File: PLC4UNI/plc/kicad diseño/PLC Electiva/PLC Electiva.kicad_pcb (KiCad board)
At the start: 2 copper layers, 102.4 x 83.1 mm, 177 parts, among them J1 Conn_02x08_Odd_Even, K1 G5V-1, K2 G5V-1, Q1 NCE60P04R, Q2 ZXMS6004FFQTA, Q3 ZXMS6004FFQTA, Q4 ZXMS6004FFQTA, Q5 ZXMS6004FFQTA, SW1 TS-1088-AR02016, U1 ESP32-S3-WROOM-1, U10 ADS1115IDGS, U11 AT3H4B-CUH-S, U12 AT3H4B-CUH-S, U13 LK1802, U14 AT3H4B-CUH-S, U15 MAX31856MUD+, U16 BL0942, U17 B0303S-1WR3_C7465185, U18 ISO7021DR, U2 AT3H4B-CUH-S, U3 AP63203WU, U4 RS485-PROTECT, U5 AT3H4B-CUH-S, U6 AT3H4B-CUH-S, U7 GP8211S-TC50-EW, U8 GP8302-TC50-EW, U9 BTS723GWXUMA1

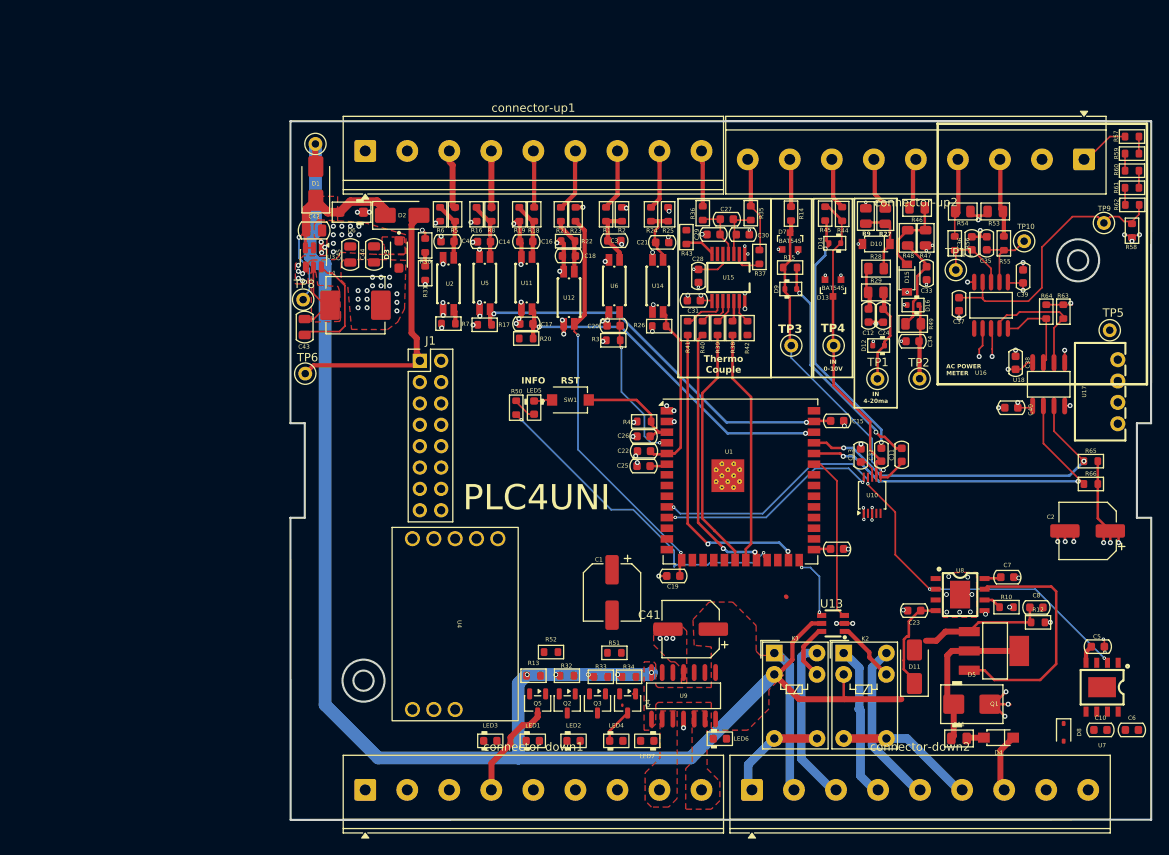
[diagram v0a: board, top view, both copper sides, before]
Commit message: Tamaños correctos
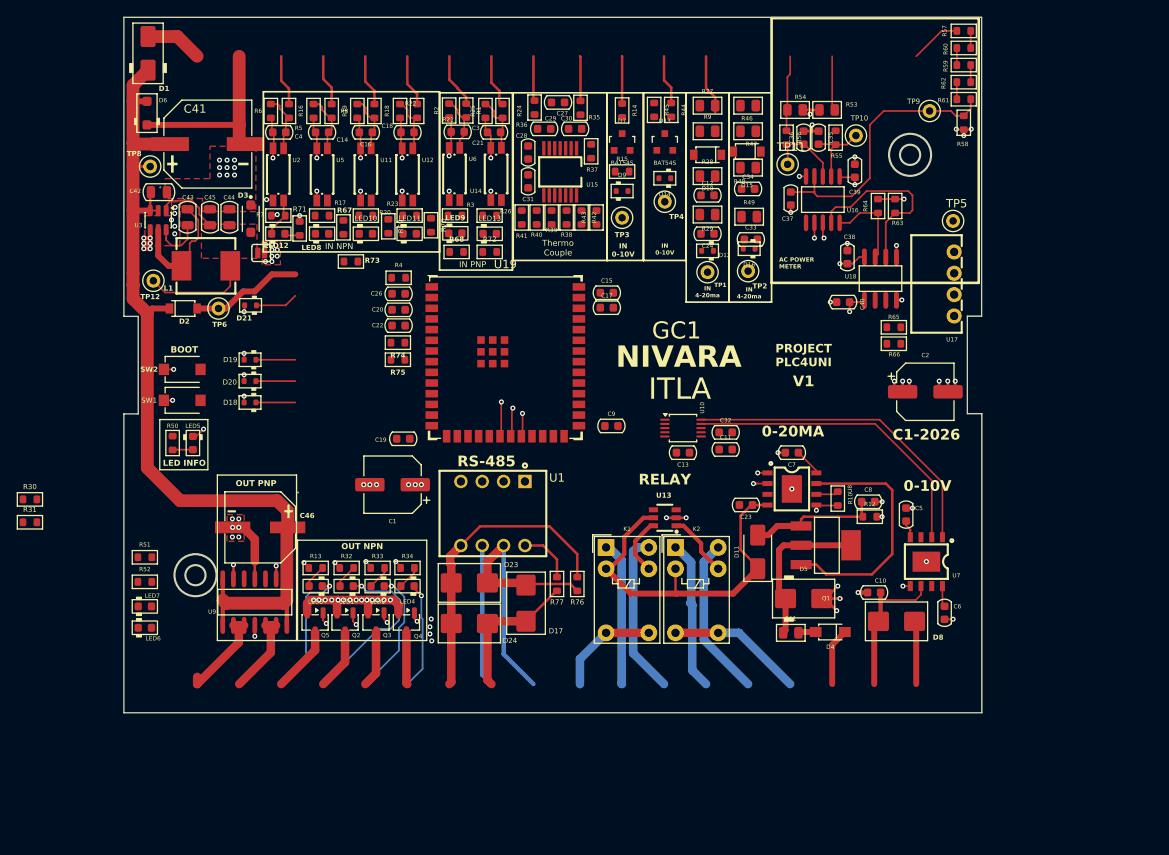
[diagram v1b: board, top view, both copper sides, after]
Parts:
- removed C25: 100nf, Capacitor_SMD_AKL:C_0603_1608Metric
- removed J1: Conn_02x08_Odd_Even, Connector_PinHeader_2.54mm:PinHeader_2x08_P2.54mm_Vertical
- removed TP7: TestPoint_Hole1, 4ms_TestPoint:TestPoint_WireHole
- removed U4: RS485-PROTECT, MG_footprints:RS-485-PROTECT
- removed connector-down1, connector-down2, connector-up1, connector-up2: Screw_Terminal_9_P5.00mm, TerminalBlock_Phoenix:TerminalBlock_Phoenix_PT-1,5-9-5.0-H_1x09_P5.00mm_Horizontal
- added C46: 100uF, EasyEDA:CAP-SMD_BD8.0-L8.3-W8.3-FD, F.Cu at (76.5, 95.8)
- added D17: SMBJ12CA, Diode_SMD_AKL:D_SMB_TVS, F.Cu at (108.1, 104.8)
- added D18: ESD5Z3.3T, Diode_SMD_AKL:D_SOD-523, F.Cu at (75.3, 80.9)
- added D19: ESD5Z3.3T, Diode_SMD_AKL:D_SOD-523, F.Cu at (75.3, 75.8)
- added D20: ESD5Z3.3T, Diode_SMD_AKL:D_SOD-523, F.Cu at (75.3, 78.4)
- added D21: ESD5Z3.3T, Diode_SMD_AKL:D_SOD-523, F.Cu at (75.4, 69.4)
- added D23: SMBJ6.5CA, Diode_SMD_AKL:D_SMB_TVS, F.Cu at (101.4, 102.4)
- added D24: SMBJ6.5CA, Diode_SMD_AKL:D_SMB_TVS, F.Cu at (101.4, 107.2)
- added JP1: ~, SparkFun-Jumper:Jumper_2_NO, F.Cu at (76.6, 63.1)
- added LED10: LED_0603_Red, LED_SMD_AKL:LED_0603_1608Metric, F.Cu at (89.1, 60.9)
- added LED11: LED_0603_Red, LED_SMD_AKL:LED_0603_1608Metric, F.Cu at (94.3, 60.9)
- added LED12: LED_0603_Red, LED_SMD_AKL:LED_0603_1608Metric, F.Cu at (78.7, 60.9)
- added LED13: LED_0603_Red, LED_SMD_AKL:LED_0603_1608Metric, F.Cu at (103.8, 60.9)
- added LED8: LED_0603_Red, LED_SMD_AKL:LED_0603_1608Metric, F.Cu at (83.9, 60.9)
- added LED9: LED_0603_Red, LED_SMD_AKL:LED_0603_1608Metric, F.Cu at (99.7, 60.8)
- added R67: R_0603, Resistor_SMD_AKL:R_0603_1608Metric, F.Cu at (86.4, 60.1)
- added R68: R_0603, Resistor_SMD_AKL:R_0603_1608Metric, F.Cu at (99.9, 63.0)
- added R69: R_0603, Resistor_SMD_AKL:R_0603_1608Metric, F.Cu at (91.7, 60.0)
- added R70: R_0603, Resistor_SMD_AKL:R_0603_1608Metric, F.Cu at (96.8, 59.8)
- added R71: R_0603, Resistor_SMD_AKL:R_0603_1608Metric, F.Cu at (81.2, 60.2)
- added R72: R_0603, Resistor_SMD_AKL:R_0603_1608Metric, F.Cu at (103.8, 63.0)
- added R73: 0R, Resistor_SMD_AKL:R_0603_1608Metric, F.Cu at (87.3, 64.2)
- added R74: 0R, Resistor_SMD_AKL:R_0603_1608Metric, F.Cu at (92.9, 73.8)
- added R75: 0R, Resistor_SMD_AKL:R_0603_1608Metric, F.Cu at (92.9, 75.8)
- added R76: 1K, Resistor_SMD_AKL:R_0603_1608Metric, F.Cu at (114.2, 102.5)
- added R77: 1K, Resistor_SMD_AKL:R_0603_1608Metric, F.Cu at (111.8, 102.5)
- added SW2: TS-1088-AR02016, EasyEDA:SW-SMD_L3.9-W3.0-P4.45, F.Cu at (67.2, 80.7)
- added TP12: TestPoint_Hole1, 4ms_TestPoint:TestPoint_WireHole, F.Cu at (63.8, 66.4)
- added U19: ESP32-S3-WROOM-1, Espressif:ESP32-S3-WROOM-1U, F.Cu at (105.7, 75.4)
- C41: value 47UF -> 220uF; footprint Capacitor_SMD:CP_Elec_6.3x7.7 -> EasyEDA:CAP-SMD_BD10.0-L10.3-W10.3-LS11.3-FD
- D1: value SS14 -> MBRA340T; footprint Diode_SMD:D_SMA -> Diode_SMD_AKL:D_SMA
- D2: value SS14 -> 1N5819HW-7-F; footprint Diode_SMD:D_SMA -> EasyEDA:SOD-123_L2.7-W1.6-LS3.7-RD
- D8: value SD12_SOD323 -> SMBJ12CA; footprint Diode_SMD:D_SOD-323 -> Diode_SMD_AKL:D_SMB_TVS
- L1: value 10uH -> APH0630T4R7M; footprint Inductor_SMD:L_APV_APH0630 -> EasyEDA:IND-SMD_L7.0-W6.6_APH0630
- R30, R31: value R_0603 -> 10K
- R4: value 22K -> 1K
- U1: value ESP32-S3-WROOM-1 -> TD301M485_C5451847; footprint RF_Module:ESP32-S3-WROOM-1U -> EasyEDA:COMM-TH_TD301M485
- moved C41 81.4 mm to (70.3, 50.2), turned to 0 degrees
- moved LED6 69.7 mm to (62.8, 107.7)
- moved LED7 61.9 mm to (62.8, 105.2), turned to 0 degrees
- moved R51 57.0 mm to (62.8, 99.3)
- moved R30 55.9 mm to (49.1, 92.4), turned to 0 degrees
- moved R31 55.6 mm to (49.1, 95.2), turned to 0 degrees
- moved U9 52.2 mm to (75.9, 104.7)
- moved R52 49.0 mm to (62.8, 102.3)
- moved SW1 46.3 mm to (67.2, 77.0), turned to 0 degrees
- moved R50 41.1 mm to (66.1, 85.7), turned to 90 degrees
- moved LED5 40.8 mm to (68.5, 85.7)
- moved C19 36.0 mm to (93.5, 85.2)
- moved R4 33.8 mm to (93.0, 66.1), turned to 0 degrees
- moved C26 33.7 mm to (93.0, 68.0)
- moved C22 32.8 mm to (93.0, 71.8)
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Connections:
- C14 pad 2: +24V -> VDC
- C16 pad 2: +24V -> VDC
- C18 pad 2: +24V -> VDC
- C23 pad 1: +24V -> VDC
- C4 pad 2: +24V -> VDC
- C41 pad 1: +24V -> VDC
- C42 pad 1: /PowerSupply/vdc_in -> VDC
- C44 pad 1: +3.3V -> /PowerSupply/ps_out
- C45 pad 1: +3.3V -> /PowerSupply/ps_out
- C5 pad 1: +24V -> VDC
- D1 pad 1: /PowerSupply/vdc_in -> VDC
- D11 pad 1: +24V -> VDC
- D2 pad 1: /PowerSupply/vdc_in -> VDC
- D3 pad A: +3.3V -> /PowerSupply/ps_out
- D6 pad 2: /PowerSupply/vdc_in -> VDC
- K1 pad 2: +24V -> VDC
- K2 pad 2: +24V -> VDC
- L1 pad 2: +3.3V -> /PowerSupply/ps_out
- R13 pad 1: +24V -> +3.3V
- R16 pad 1: +24V -> VDC
- R19 pad 1: +24V -> VDC
- R22 pad 1: +24V -> VDC
- R30 pad 1: +24V -> +3.3V
- R30 pad 2: /control/IN_VDC_ADC -> /control/RS485-RX
- R31 pad 1: /control/IN_VDC_ADC -> +3.3V
- R31 pad 2: GND -> /control/RS485-TX
- R32 pad 1: +24V -> +3.3V
- R33 pad 1: +24V -> +3.3V
- R34 pad 1: +24V -> +3.3V
- R38 pad 2: /control/mosi -> /control/SPI_MOSI
- R39 pad 2: /control/miso -> /control/SPI_MISO
- R4 pad 1: /control/EN -> +3.3V
- R4 pad 2: +3.3V -> /control/EN
- R40 pad 2: /control/clk -> /control/SPI_CLK
- R42 pad 2: /control/TC//FAULT -> /control/TC_FAULT
- R6 pad 1: +24V -> VDC
- SW1 pad 1: /control/EN -> GND
- SW1 pad 2: GND -> /control/IN_NPN1
- TP8 pad 1: /PowerSupply/vdc_in -> VDC
- U1 pad 1: GND -> /control/RS485-RX
- U1 pad 2: +3.3V -> /control/RS485-TX
- U1 pad 3: /control/EN -> GND
- U1 pad 4: /control/IN_PNP1 -> +3.3V
- U1 pad 5: /control/IN_PNP2 -> /control/CON_RS485_G
- U1 pad 6: /control/IN_VDC_ADC -> /control/CON_RS485_B
- U1 pad 7: /control/acc_cs -> /control/CON_RS485_A
- U1 pad 8: /control/GPIO1 -> Net-(U1-VO)
- U10 pad 10: /control/i2c_scl -> /control/I2C_SCK
- U10 pad 9: /control/i2c_sda -> /control/I2C_SDA
- U11 pad 2: +24V -> VDC
- U12 pad 2: +24V -> VDC
- U13 pad 5: +24V -> VDC
- U2 pad 2: +24V -> VDC
- U3 pad 1: +3.3V -> /PowerSupply/ps_out
- U3 pad 2: /PowerSupply/vdc_in -> VDC
- U3 pad 3: /PowerSupply/vdc_in -> VDC
- U5 pad 2: +24V -> VDC
- U7 pad 1: /control/i2c_scl -> /control/I2C_SCK
- U7 pad 2: /control/i2c_sda -> /control/I2C_SDA
- U7 pad 4: +24V -> VDC
- U8 pad 1: /control/i2c_scl -> /control/I2C_SCK
- U8 pad 2: /control/i2c_sda -> /control/I2C_SDA
- U8 pad 4: +24V -> VDC
- U9 pad 1: +24V -> VDC
- U9 pad 14: +24V -> VDC
- U9 pad 7: +24V -> VDC
- U9 pad 8: +24V -> VDC
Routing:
- net +24V: track 216.0 -> 6.82 mm, vias 16 -> 0
- net VDC: track 0.00 -> 179.3 mm, vias 0 -> 4
- net /control/i2c_sda: track 69.9 -> 0.00 mm, vias 4 -> 0
- net /control/IN_NPN4: track 48.7 -> 0.00 mm, vias 2 -> 0
- net /control/IN_NPN2: track 48.4 -> 0.00 mm, vias 2 -> 0
- net GND: track 60.5 -> 107.1 mm, vias 97 -> 78
- net /control/EMRX: track 44.9 -> 0.00 mm, vias 2 -> 0
- net /control/IN_NPN3: track 42.6 -> 0.00 mm, vias 2 -> 0
- net /control/EM_TX: track 42.5 -> 0.00 mm, vias 2 -> 0
- net /control/IN-0-10V/OUT3V: track 40.0 -> 0.00 mm, vias 1 -> 0
- net /control/LED_INFO: track 39.8 -> 0.00 mm, vias 2 -> 0
- net /control/I2C_SCK: track 0.00 -> 39.5 mm, vias 0 -> 1
- net /control/I2C_SDA: track 0.00 -> 38.6 mm, vias 0 -> 1
- net /control/TEMP_CS: track 37.3 -> 0.00 mm, vias 2 -> 0
- net /control/IN-0-10V1/OUT3V: track 36.6 -> 0.00 mm
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- added copper zone on F.Cu, net /PowerSupply/ps_out
- removed copper zone on F.Cu, net +24V
- removed copper zone on F.Cu, net /PowerSupply/sw
- removed copper zone on F.Cu, net /control/CON_OUT_PNP1
- removed copper zone on F.Cu, net /control/CON_OUT_PNP2
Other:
- board size 102.4 x 83.1 mm -> 102 x 82.7 mm
- board text added: "+3.3V"
- board text added: "+5"
- board text added: "0-10V"
- board text added: "0-20MA"
- board text added: "BOOT"
- board text added: "C1-2026"
- board text added: "GC1"
- board text added: "GND"
- board text added: "I2C_SCK"
- board text added: "I2C_SDA"
- board text added: "IN NPN"
- board text added: "IN PNP"
- board text added: "ITLA"
- board text added: "LCD_CS"
- board text added: "LCD_EN"
- board text added: "LED INFO"
- board text added: "NIVARA"
- board text added: "OUT NPN"
- board text added: "OUT PNP"
- board text added: "PROJECT PLC4UNI"
- board text added: "RELAY"
- board text added: "RESET"
- board text added: "RS-485"
- board text added: "SD_CS"
- board text added: "SPI_CLK"
- board text added: "SPI_MISO"
- board text added: "SPI_MOSI"
- board text added: "TP_INT"
- board text added: "USB+"
- board text added: "USB-"
- board text added: "V1"
- board text removed: "INFO"
- board text removed: "PLC4UNI"
- board text removed: "RST"
